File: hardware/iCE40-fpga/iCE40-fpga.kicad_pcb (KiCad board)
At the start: 4 copper layers, 50 x 22.9 mm, 61 parts, among them J1 USB_B_Micro, J2 JST_PH, J3 Feather, Q1 DMP2045U, U1 MCP73831-2-OT, U2 W25Q32JVZP, U3 AP2112K-3.3, U5 AP2112K-1.2, U6 ICE40UP5K-SG48ITR, U7 93C46B, U8 FT2232H, X1 DSC6101CI1A

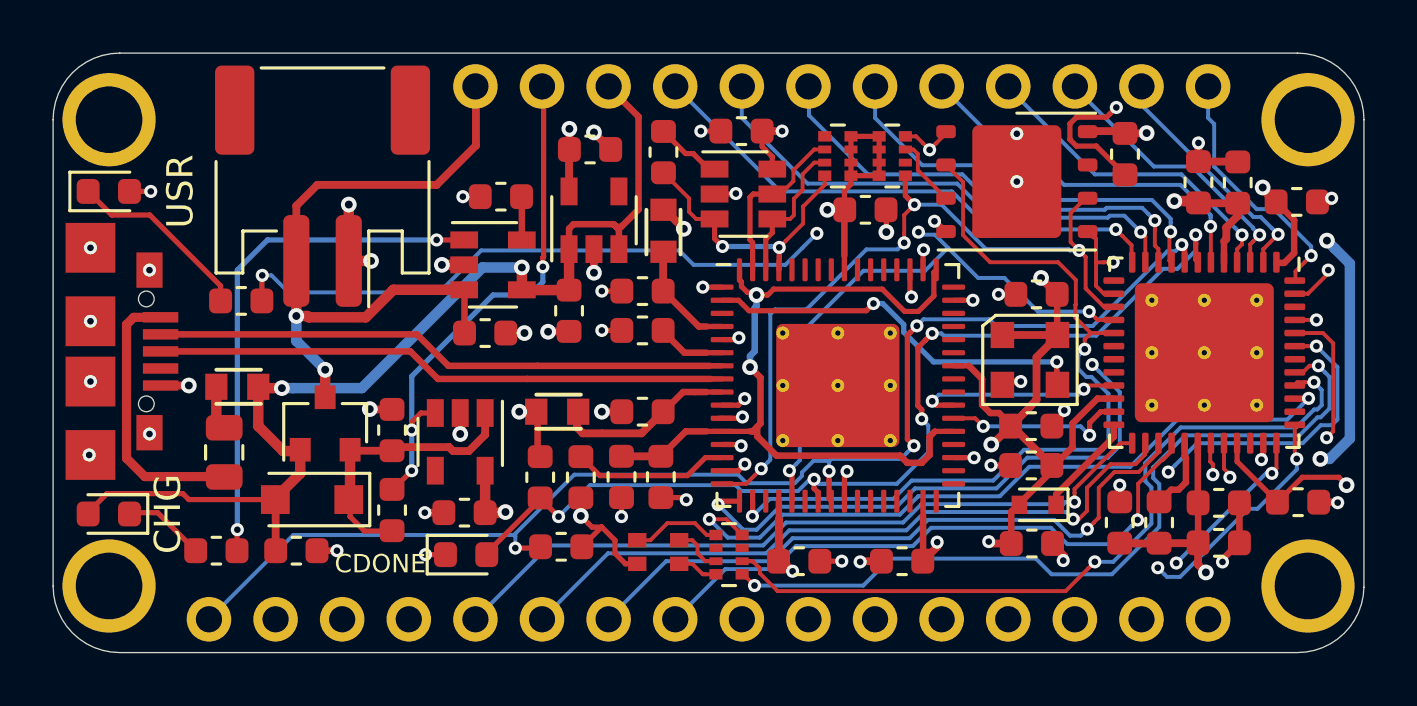
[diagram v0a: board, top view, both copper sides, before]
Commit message: cleaned up routing
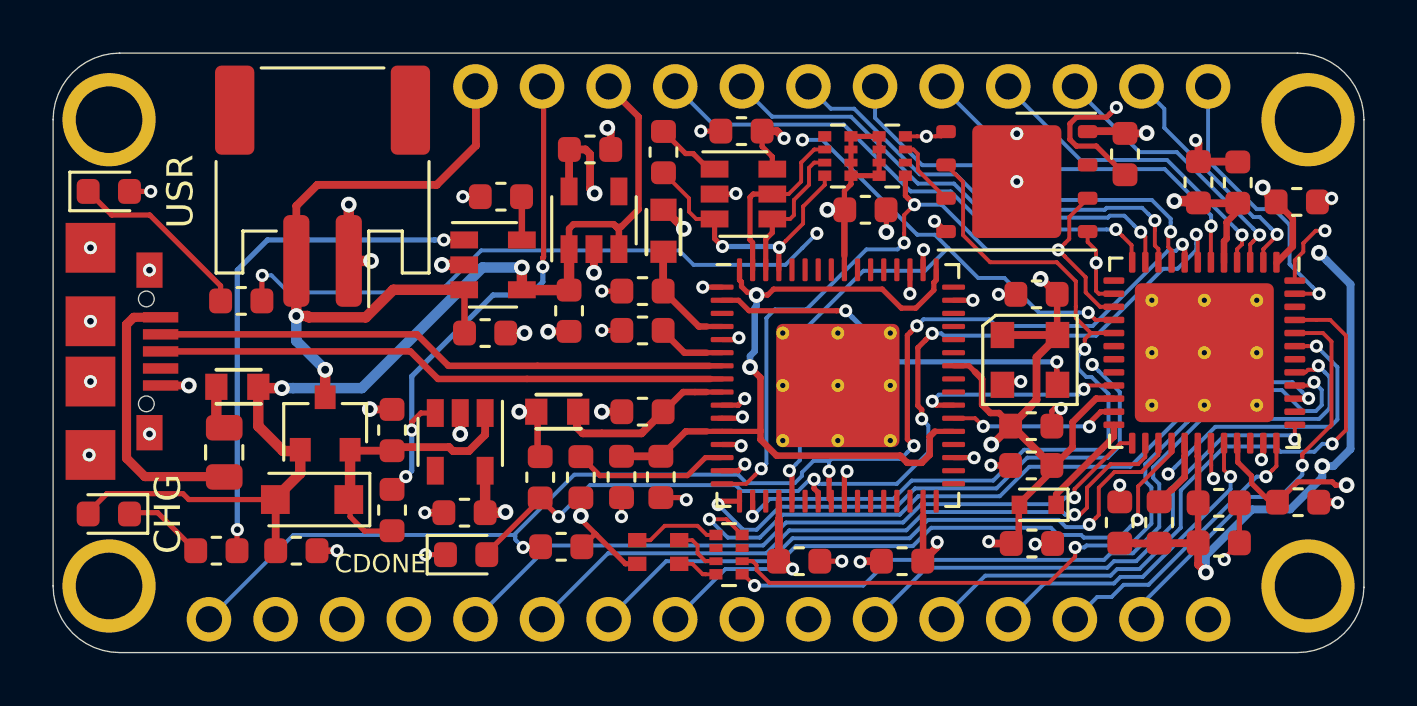
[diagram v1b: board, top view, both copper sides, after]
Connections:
- U6 pad 31: /IO4 -> /IO5
- U6 pad 32: /IO5 -> /IO8
- U6 pad 36: /IO6 -> /IO9
- U6 pad 37: /IO7 -> /IO6
- U6 pad 43: /IO8 -> /IO4
- U6 pad 45: /IO9 -> /IO7
- U6 pad 47: /nLED -> /IO11
- U6 pad 48: /IO11 -> /nLED
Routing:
- net /IO4: track 21.9 -> 30.3 mm, vias 1 -> 2
- net /IO8: track 20.0 -> 12.4 mm, vias 2 -> 1
- net /IO7: track 17.9 -> 25.2 mm, vias 2 -> 1
- net /ICE_SS: track 27.8 -> 34.7 mm
- net /IO9: track 17.6 -> 11.3 mm
- net /nLED: track 49.8 -> 48.2 mm
- net /IO6: track 18.9 -> 20.4 mm, vias 2 -> 1
- net /IO11: track 9.67 -> 11.0 mm
- net /IO10: track 17.0 -> 15.8 mm
- net /nLED_GREEN: track 29.1 -> 30.1 mm
- net /nLED_BLUE: track 27.4 -> 28.3 mm
- net +1V2: track 65.0 -> 64.3 mm
- net /IO18: track 19.5 -> 18.8 mm
- net /FLASH_MOSI|IO0: track 29.4 -> 28.8 mm
- net /IO17: track 17.7 -> 17.0 mm
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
